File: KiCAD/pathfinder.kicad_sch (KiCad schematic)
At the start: 7 parts, among them SW1 SW_Push, SW2 SW_Push, SW3 SW_Push, U1 MOUDLE-SEEEDUINO-XIAO

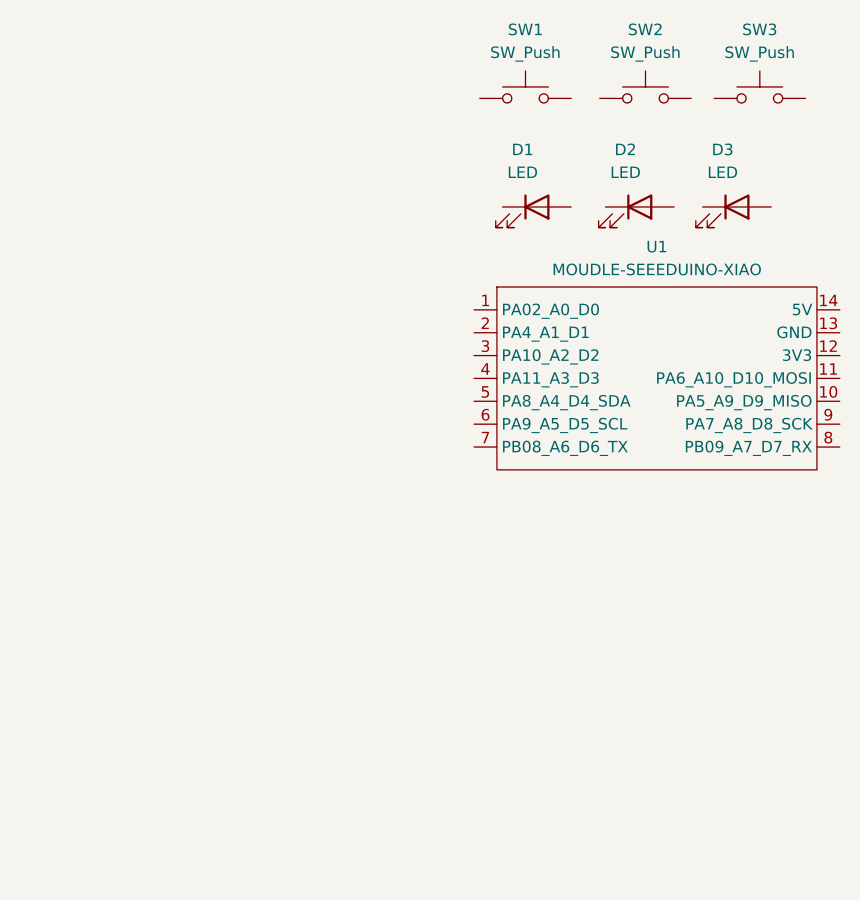
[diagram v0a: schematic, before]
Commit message: schematic tutorial
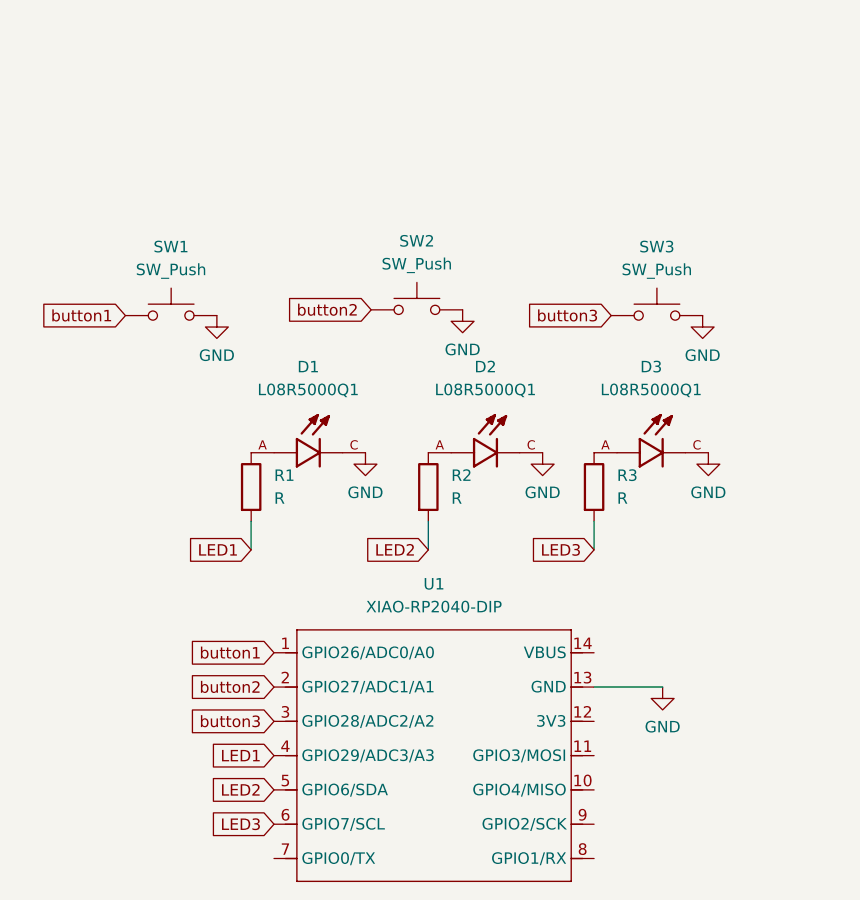
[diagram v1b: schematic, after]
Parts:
- removed D1, D2, D3: LED, symbol Device:LED
- removed U1: MOUDLE-SEEEDUINO-XIAO, symbol XIAO_RP2040:MOUDLE-SEEEDUINO-XIAO
- added D1, D2, D3: L08R5000Q1, L08R5000Q1:LEDRD254W57D500H1070, symbol L08R5000Q1:L08R5000Q1
- added R1, R2, R3: R, symbol Device:R
- added U1: XIAO-RP2040-DIP, Module:MOUDLE14P-XIAO-DIP-SMD, symbol Seeed_Studio_XIAO_Series:XIAO-RP2040-DIP
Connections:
- net button2: now reaches SW2.1
- net button2: now also U1.2 (GPIO27/ADC1/A1)
- net GND: now reaches SW2.2
- net GND: now also SW1.2, SW3.2, D1.C, D2.C, D3.C, U1.13 (GND)
- net button1: now reaches SW1.1
- net button1: now also U1.1 (GPIO26/ADC0/A0)
- net button3: now reaches SW3.1
- net button3: now also U1.3 (GPIO28/ADC2/A2)
- new net: D1.A, R1.1
- new net: D3.A, R3.1
- new net: D2.A, R2.1
- new net LED1: R1.2, U1.4 (GPIO29/ADC3/A3)
- new net LED2: R2.2, U1.5 (GPIO6/SDA)
- new net LED3: R3.2, U1.6 (GPIO7/SCL)
